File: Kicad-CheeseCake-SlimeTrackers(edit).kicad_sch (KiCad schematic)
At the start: 15 parts, among them J2 USB_C-16p, Q1 UMH3N, SW1 SW_SPDT, U2 TP4057, U3 CH340K

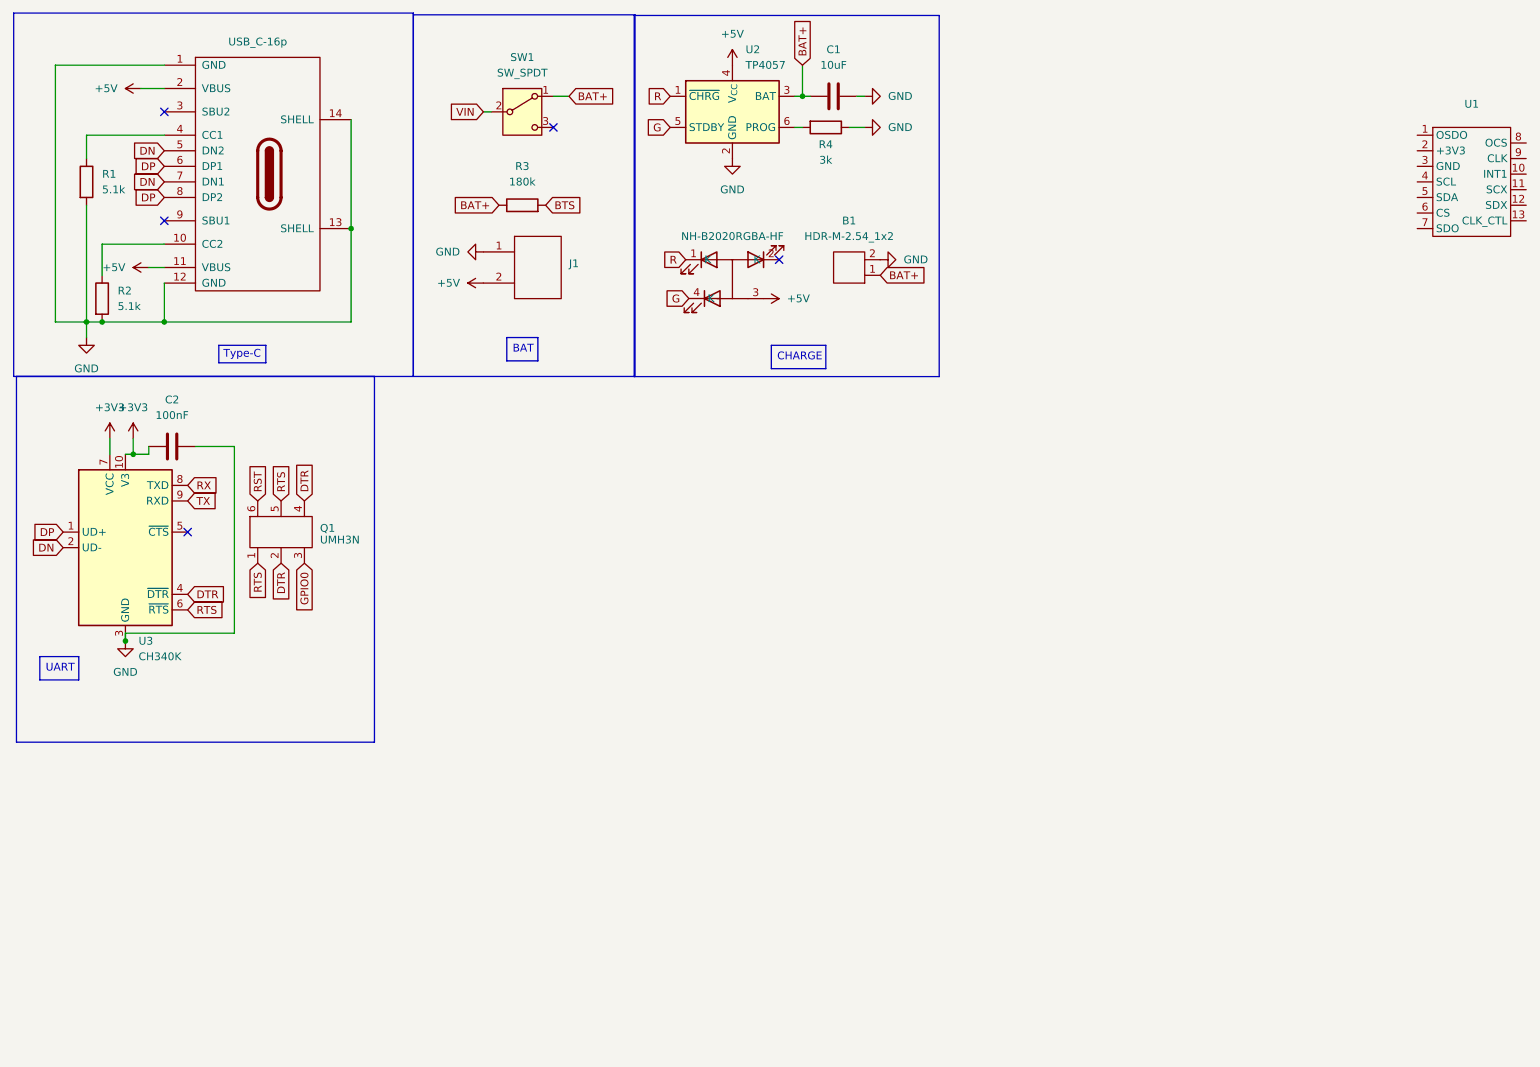
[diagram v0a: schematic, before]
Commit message: updt
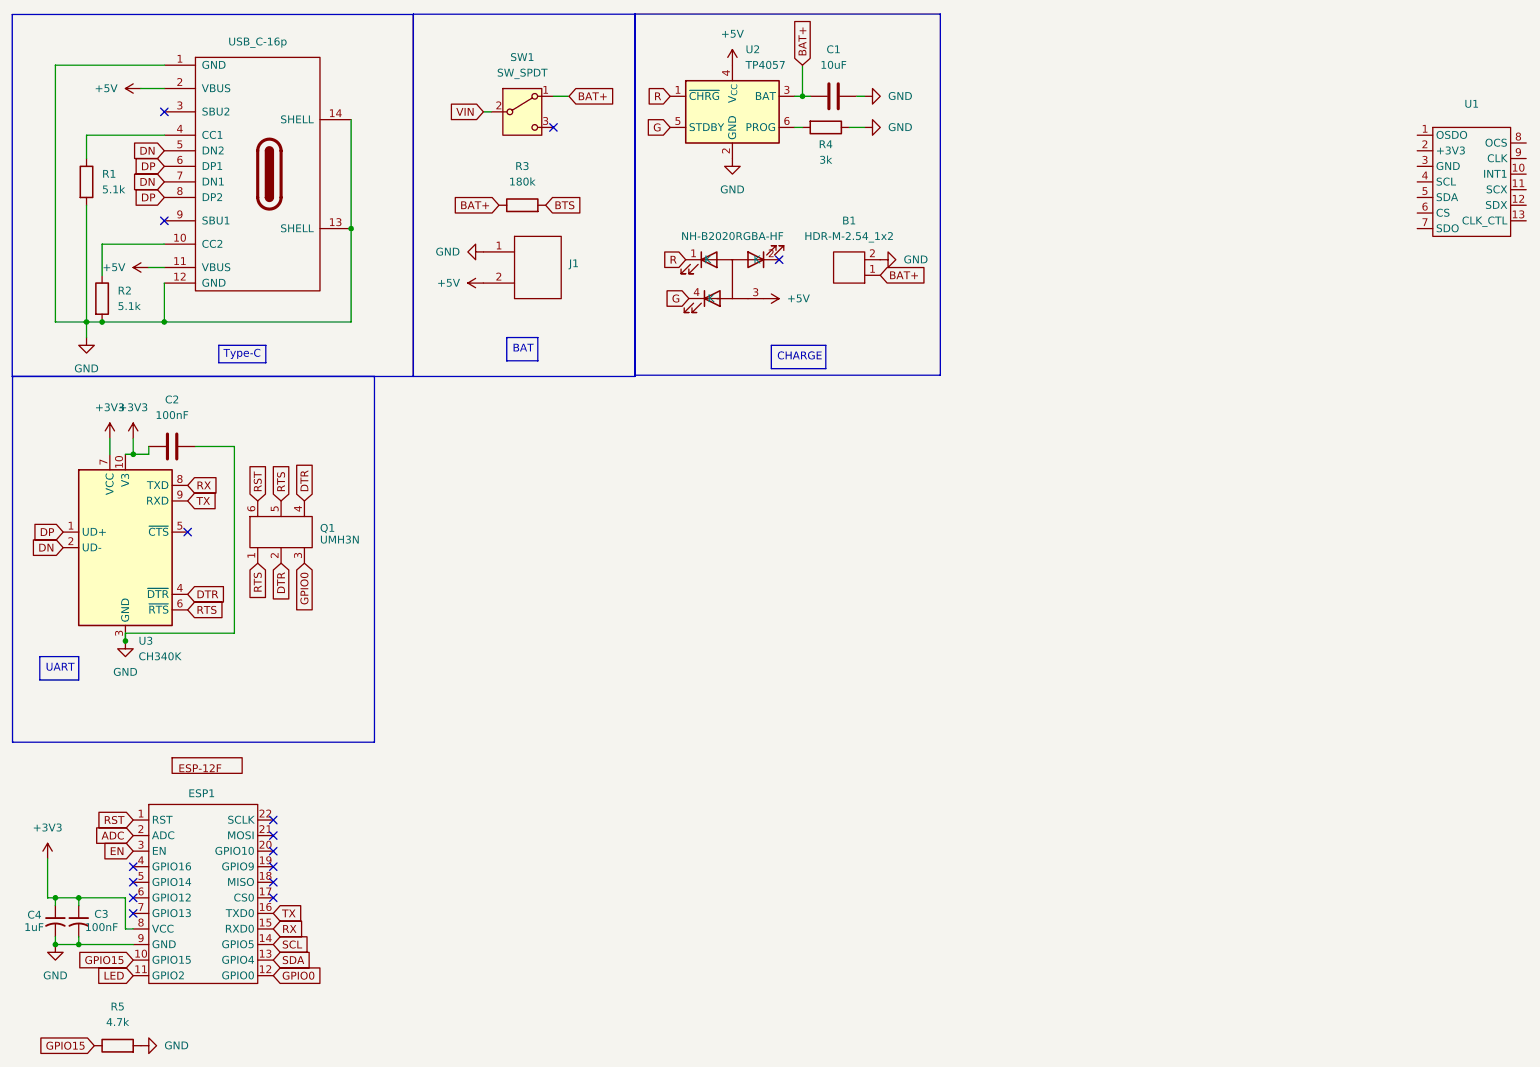
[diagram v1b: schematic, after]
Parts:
- added C3: 100nF, symbol Device:C_Small_US
- added C4: 1uF, symbol Device:C_Small_US
- added ESP1: ~, symbol _symbolsslime:ESP12F_edit
- added R5: 4.7k, symbol Device:R
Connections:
- net +3V3: now also C3.1, C4.1, ESP1.8 (VCC)
- net GND: now also C3.2, C4.2, ESP1.9 (GND), R5.2
- net GPIO0: now also ESP1.12 (GPIO0)
- net RST: now also ESP1.1 (RST)
- net RX: now also ESP1.15 (RXD0)
- net TX: now also ESP1.16 (TXD0)
- new net ADC: ESP1.2 (ADC)
- new net EN: ESP1.3 (EN)
- new net GPIO15: ESP1.10 (GPIO15), R5.1
- new net LED: ESP1.11 (GPIO2)
- new net SCL: ESP1.14 (GPIO5)
- new net SDA: ESP1.13 (GPIO4)
- no-connect marks 5 -> 15
